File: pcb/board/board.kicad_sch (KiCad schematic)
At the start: 31 parts, among them J1 USB_C_Receptacle_USB2.0_14P, J2 Conn_01x03, SW1 SW_Push, U1 RP2040, U2 NCP1117-3.3_SOT223, U3 W25Q128JVS, Y1 12MHz

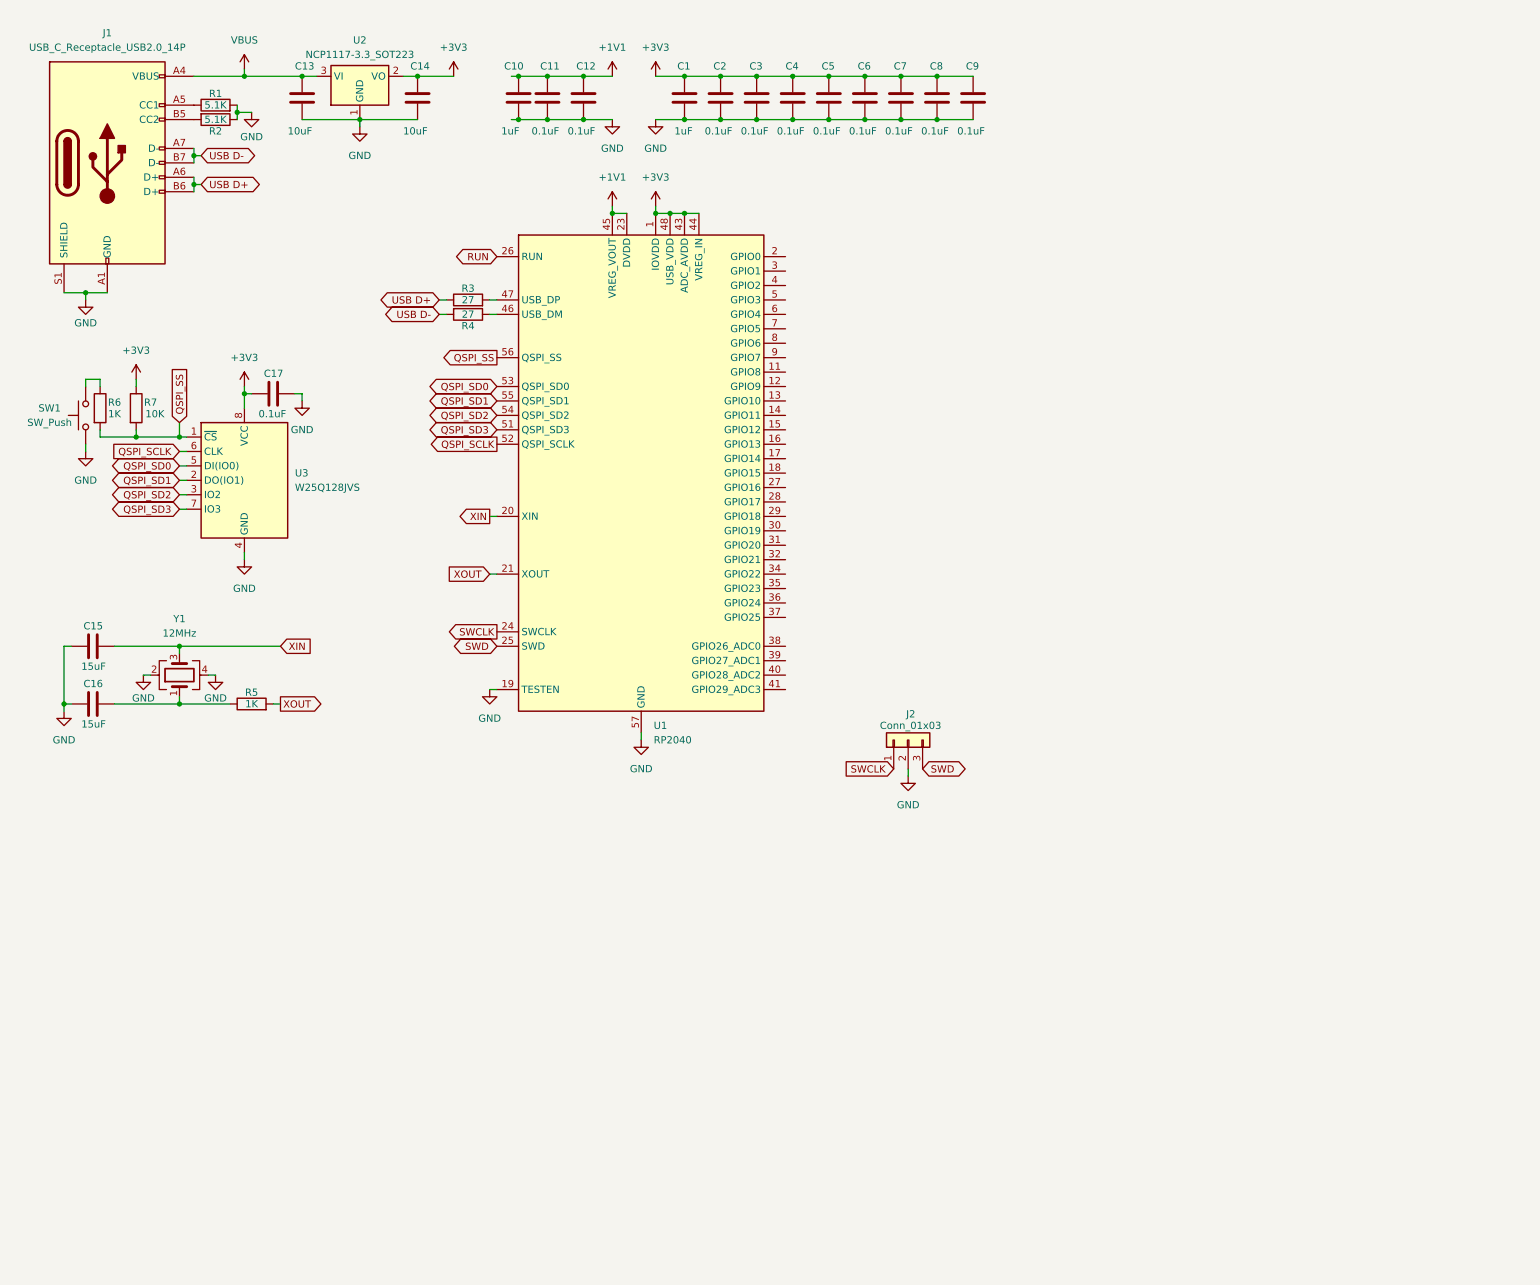
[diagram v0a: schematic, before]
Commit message: 08012026 - tons of schematic work!
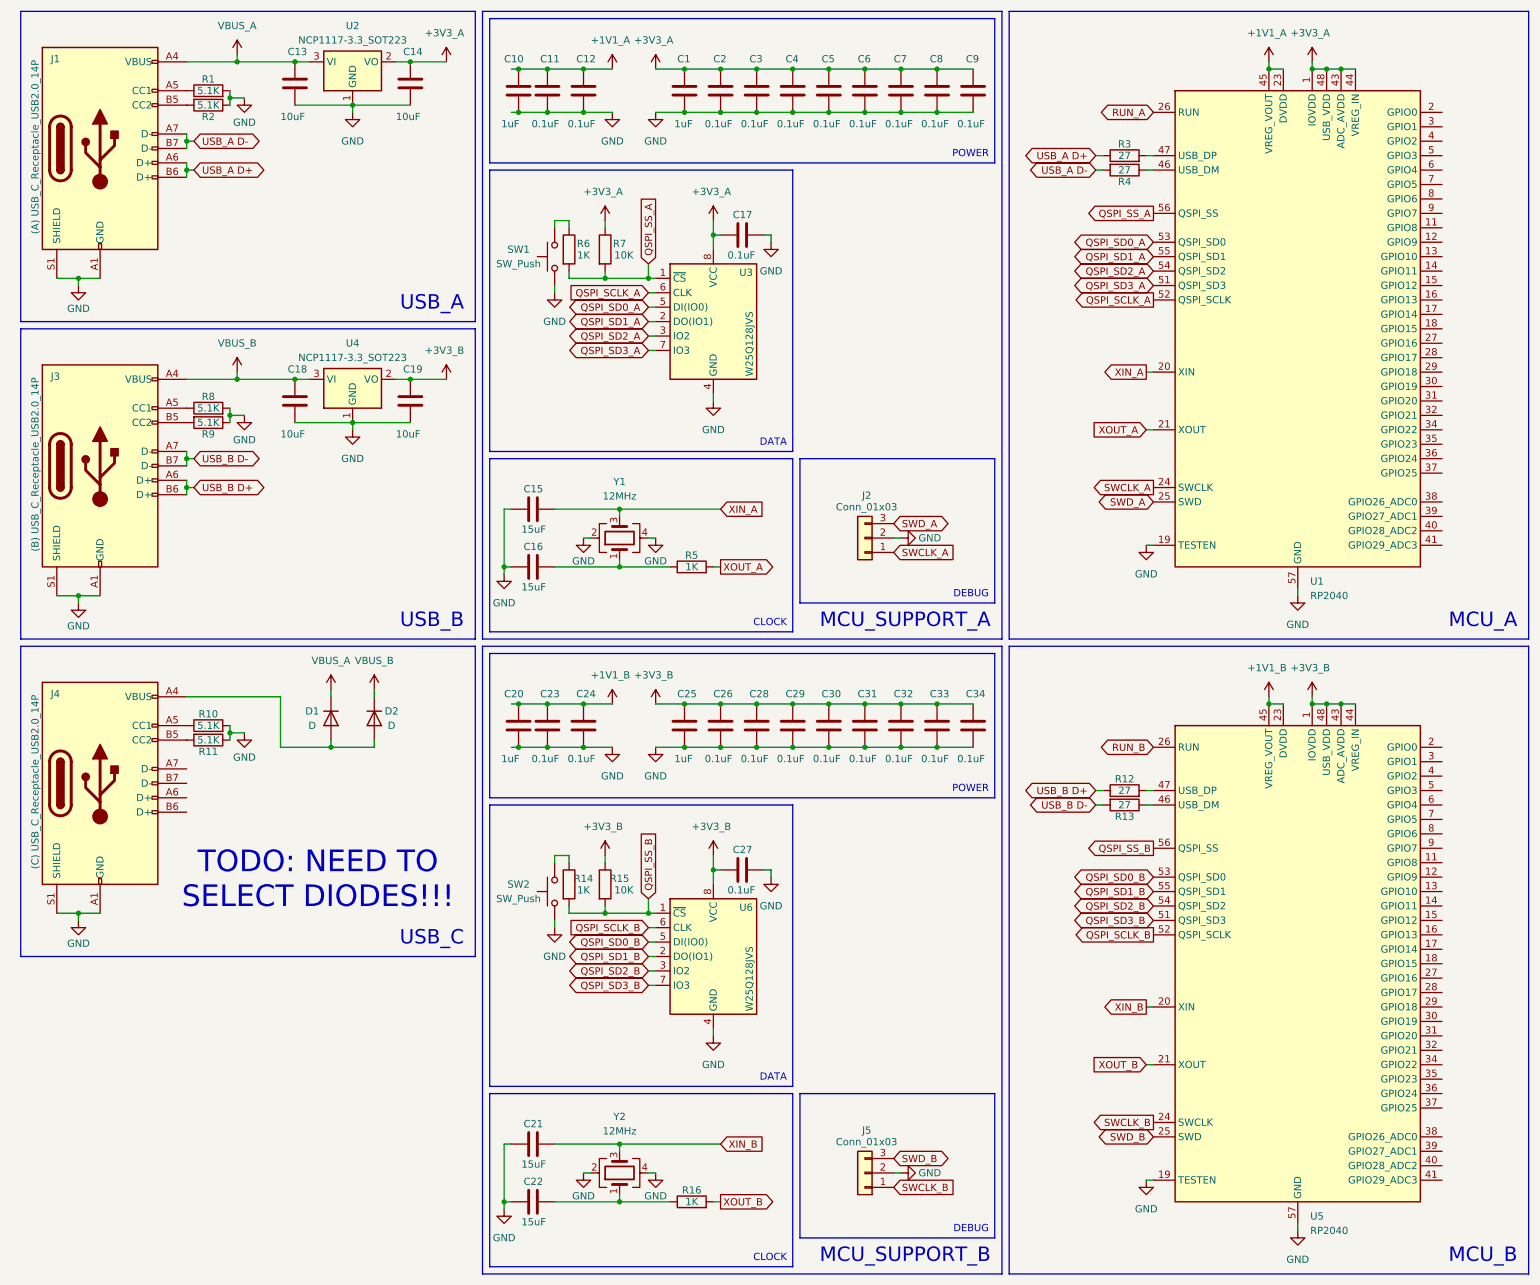
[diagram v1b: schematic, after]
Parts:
- added C18, C19: 10uF, symbol Device:C
- added C20, C25: 1uF, symbol Device:C
- added C21, C22: 15uF, symbol Device:C
- added C23, C24, C26, C27, C28, C29, C30, C31, C32, C33, C34: 0.1uF, symbol Device:C
- added D1, D2: D, symbol Device:D
- added J3: (B) USB_C_Receptacle_USB2.0_14P, symbol Connector:USB_C_Receptacle_USB2.0_14P
- added J4: (C) USB_C_Receptacle_USB2.0_14P, symbol Connector:USB_C_Receptacle_USB2.0_14P
- added J5: Conn_01x03, symbol Connector_Generic:Conn_01x03
- added R10, R11, R8, R9: 5.1K, symbol Device:R
- added R12, R13: 27, symbol Device:R
- added R14, R16: 1K, symbol Device:R
- added R15: 10K, symbol Device:R
- added SW2: SW_Push, symbol Switch:SW_Push
- added U4: NCP1117-3.3_SOT223, Package_TO_SOT_SMD:SOT-223-3_TabPin2, symbol Regulator_Linear:NCP1117-3.3_SOT223
- added U5: RP2040, Package_DFN_QFN:QFN-56-1EP_7x7mm_P0.4mm_EP3.2x3.2mm, symbol MCU_RaspberryPi:RP2040
- added U6: W25Q128JVS, Package_SO:SOIC-8_5.23x5.23mm_P1.27mm, symbol Memory_Flash:W25Q128JVS
- added Y2: 12MHz, symbol Device:Crystal_GND24
- J1: value USB_C_Receptacle_USB2.0_14P -> (A) USB_C_Receptacle_USB2.0_14P
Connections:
- net GND: now also C18.2, C19.2, C20.2, C21.1, C22.1, C23.2, C24.2, C25.2, C26.2, C27.2, C28.2, C29.2, C30.2, C31.2, C32.2, C33.2, C34.2, J3.A1 (GND), J3.A12 (GND), J3.B1 (GND), J3.B12 (GND), J3.S1 (SHIELD), J4.A1 (GND), J4.A12 (GND), J4.B1 (GND), J4.B12 (GND), J4.S1 (SHIELD), J5.2 (Pin_2), R10.2, R11.1, R8.2, R9.1, SW2.1, U4.1 (GND), U5.19 (TESTEN), U5.57 (GND), U6.4 (GND), Y2.2, Y2.4
- net +1V1 renamed +1V1_A
- net +3V3 renamed +3V3_A
- net QSPI_SCLK renamed QSPI_SCLK_A
- net QSPI_SD0 renamed QSPI_SD0_A
- net QSPI_SD1 renamed QSPI_SD1_A
- net QSPI_SD2 renamed QSPI_SD2_A
- net QSPI_SD3 renamed QSPI_SD3_A
- net QSPI_SS renamed QSPI_SS_A
- net RUN renamed RUN_A
- net SWCLK renamed SWCLK_A
- net SWD renamed SWD_A
- net USB D+ renamed USB_A D+
- net USB D- renamed USB_A D-
- net VBUS renamed VBUS_A
- net VBUS_A: now also D1.1 (K)
- net XIN renamed XIN_A
- net XOUT renamed XOUT_A
- new net: D1.2 (A), D2.2 (A), J4.A4 (VBUS), J4.A9 (VBUS), J4.B4 (VBUS), J4.B9 (VBUS)
- new net: C22.2, R16.1, Y2.1
- new net: J4.A5 (CC1), R10.1
- new net: J4.B5 (CC2), R11.2
- new net: R14.1, SW2.2
- new net: J3.A5 (CC1), R8.1
- new net: R13.1, U5.46 (USB_DM)
- new net: R12.2, U5.47 (USB_DP)
- new net: J3.B5 (CC2), R9.2
- new net +1V1_B: C20.1, C23.1, C24.1, U5.23 (DVDD), U5.45 (VREG_VOUT), U5.50 (DVDD)
- new net +3V3_B: C19.1, C25.1, C26.1, C27.1, C28.1, C29.1, C30.1, C31.1, C32.1, C33.1, C34.1, R15.1, U4.2 (VO), U5.1 (IOVDD), U5.10 (IOVDD), U5.22 (IOVDD), U5.33 (IOVDD), U5.42 (IOVDD), U5.43 (ADC_AVDD), U5.44 (VREG_IN), U5.48 (USB_VDD), U5.49 (IOVDD), U6.8 (VCC)
- new net QSPI_SCLK_B: U5.52 (QSPI_SCLK), U6.6 (CLK)
- new net QSPI_SD0_B: U5.53 (QSPI_SD0), U6.5 (DI(IO0))
- new net QSPI_SD1_B: U5.55 (QSPI_SD1), U6.2 (DO(IO1))
- new net QSPI_SD2_B: U5.54 (QSPI_SD2), U6.3 (IO2)
- new net QSPI_SD3_B: U5.51 (QSPI_SD3), U6.7 (IO3)
- new net QSPI_SS_B: R14.2, R15.2, U5.56 (QSPI_SS), U6.1 (~{CS})
- new net RUN_B: U5.26 (RUN)
- new net SWCLK_B: J5.1 (Pin_1), U5.24 (SWCLK)
- new net SWD_B: J5.3 (Pin_3), U5.25 (SWD)
- new net USB_B D+: J3.A6 (D+), J3.B6 (D+), R12.1
- new net USB_B D-: J3.A7 (D-), J3.B7 (D-), R13.2
- new net VBUS_B: C18.1, D2.1 (K), J3.A4 (VBUS), J3.A9 (VBUS), J3.B4 (VBUS), J3.B9 (VBUS), U4.3 (VI)
- new net XIN_B: C21.2, U5.20 (XIN), Y2.3
- new net XOUT_B: R16.2, U5.21 (XOUT)
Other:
- note added: "TODO: NEED TO SELECT DIODES!!!"
- moved on the sheet: C1, C10, C11, C12, C13, C14, C15, C16, C17, C2, C3, C4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
